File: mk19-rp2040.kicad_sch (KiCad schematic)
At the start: 141 parts, among them J1 USB_C_Receptacle_USB2.0, J10 Conn_01x02, J11 Conn_01x03_Socket, J12 USB_C_Receptacle_USB2.0, J13 USB_C_Receptacle_USB2.0, J2 Conn_01x03_Socket, J3 Conn_01x02_Socket, J4 Conn_01x06_Socket, J5 Conn_01x02, J7 Conn_01x02_Socket, J8 Conn_01x02_Socket, J9 Conn_01x02_Socket, T1 Conn_01x01_Socket, T10 Conn_01x01_Socket, T11 Conn_01x01_Socket, T12 Conn_01x01_Socket, T13 Conn_01x01_Socket, T14 Conn_01x01_Socket, T15 Conn_01x01_Socket, T2 Conn_01x01_Socket, T3 Conn_01x01_Socket, T5 Conn_01x01_Socket, T6 Conn_01x01_Socket, T7 Conn_01x01_Socket, T9 Conn_01x01_Socket, U1 RP2040, U10 1N4148W_C81598, U11 1N4148W_C81598, U12 1N4148W_C81598, U13 1N4148W_C81598, U14 1N4148W_C81598, U15 1N4148W_C81598, U16 W25Q128JVSIQTR, U3 XC6210B332MR-G, U6 8_01A0_008200, U7 8_01A0_008200, U9 1N4148W_C81598, Y1 Crystal_GND24

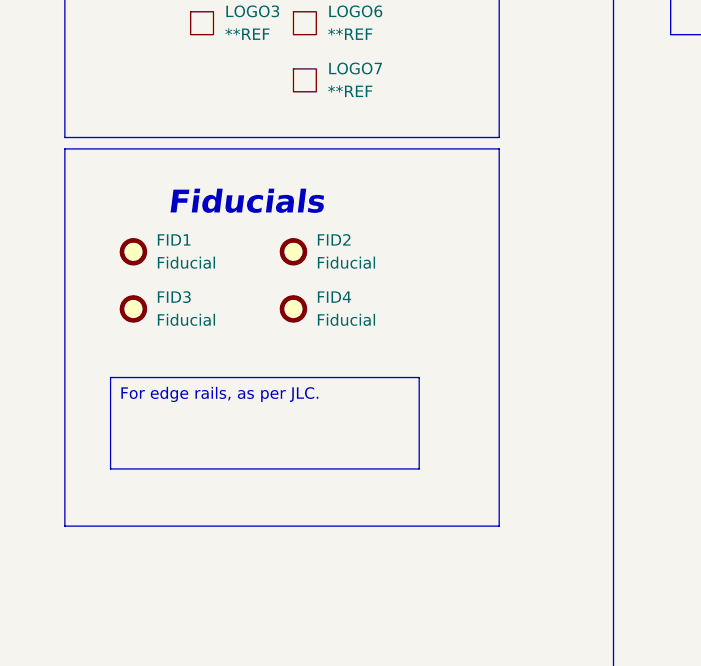
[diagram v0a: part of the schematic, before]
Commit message: getting manufacturing bits ready
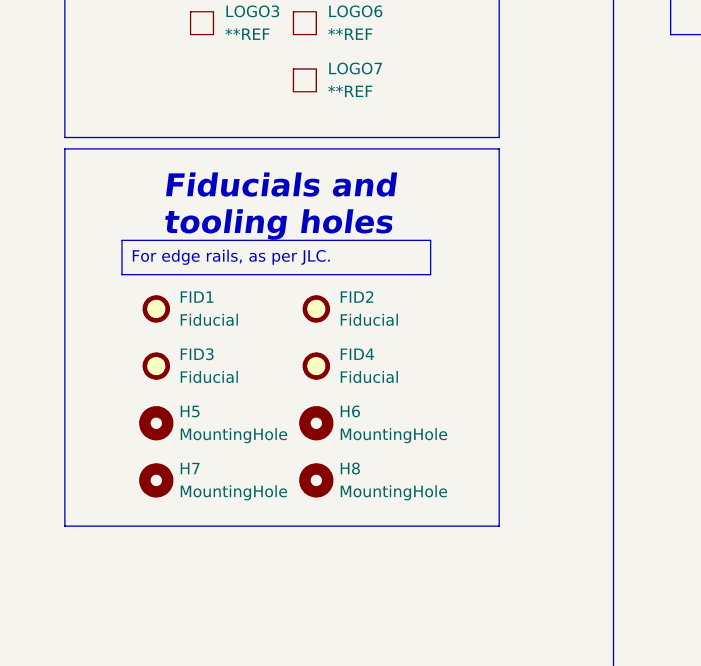
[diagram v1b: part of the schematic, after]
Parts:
- added H5, H6, H7, H8: MountingHole, MountingHole:MountingHole_2.1mm, symbol Mechanical:MountingHole
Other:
- note added: "Fiducials and tooling holes"
- note removed: "Fiducials"
- moved on the sheet: FID1, FID2, FID3, FID4
